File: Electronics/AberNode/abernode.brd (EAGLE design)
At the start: 100 x 80 mm, 12 parts, among them IC1 MCP1703CB, Y1 16MHZ, Y2 16MHZ

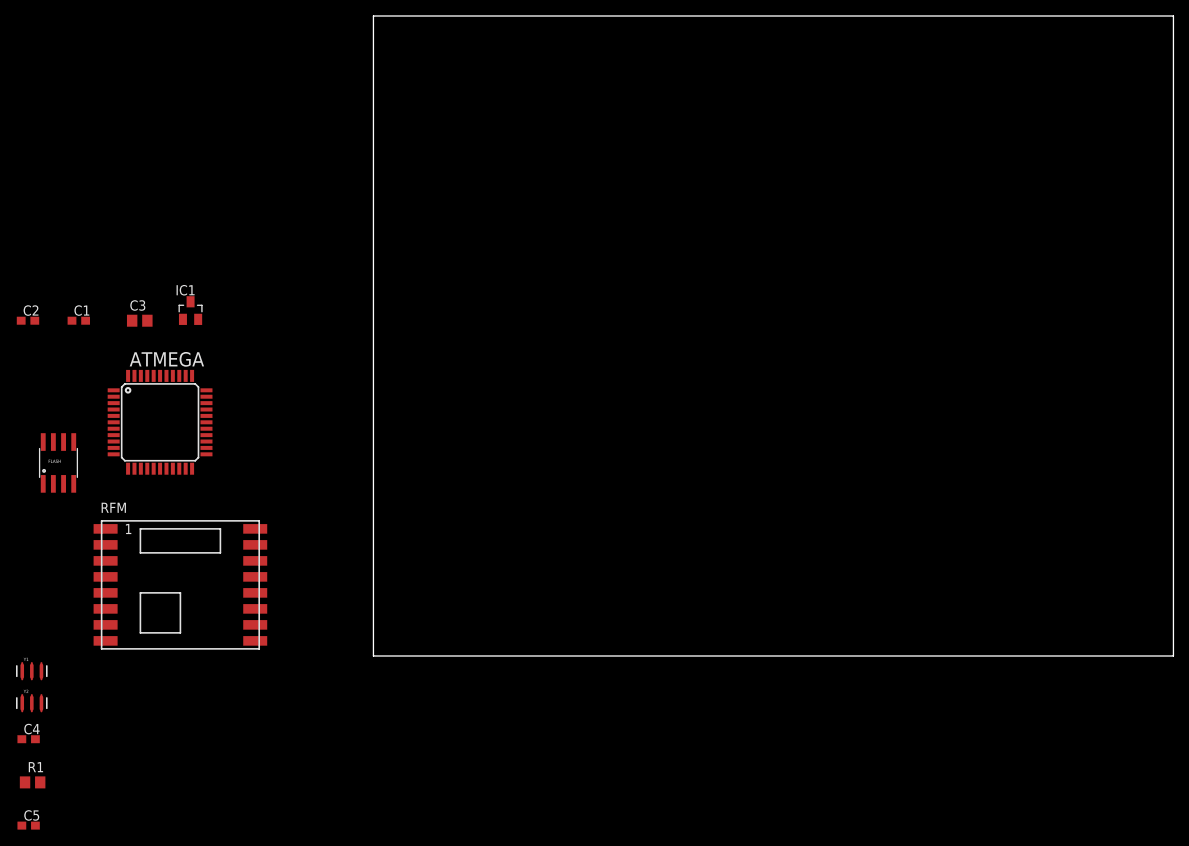
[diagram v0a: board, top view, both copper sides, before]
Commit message: Schematic Mostly Done
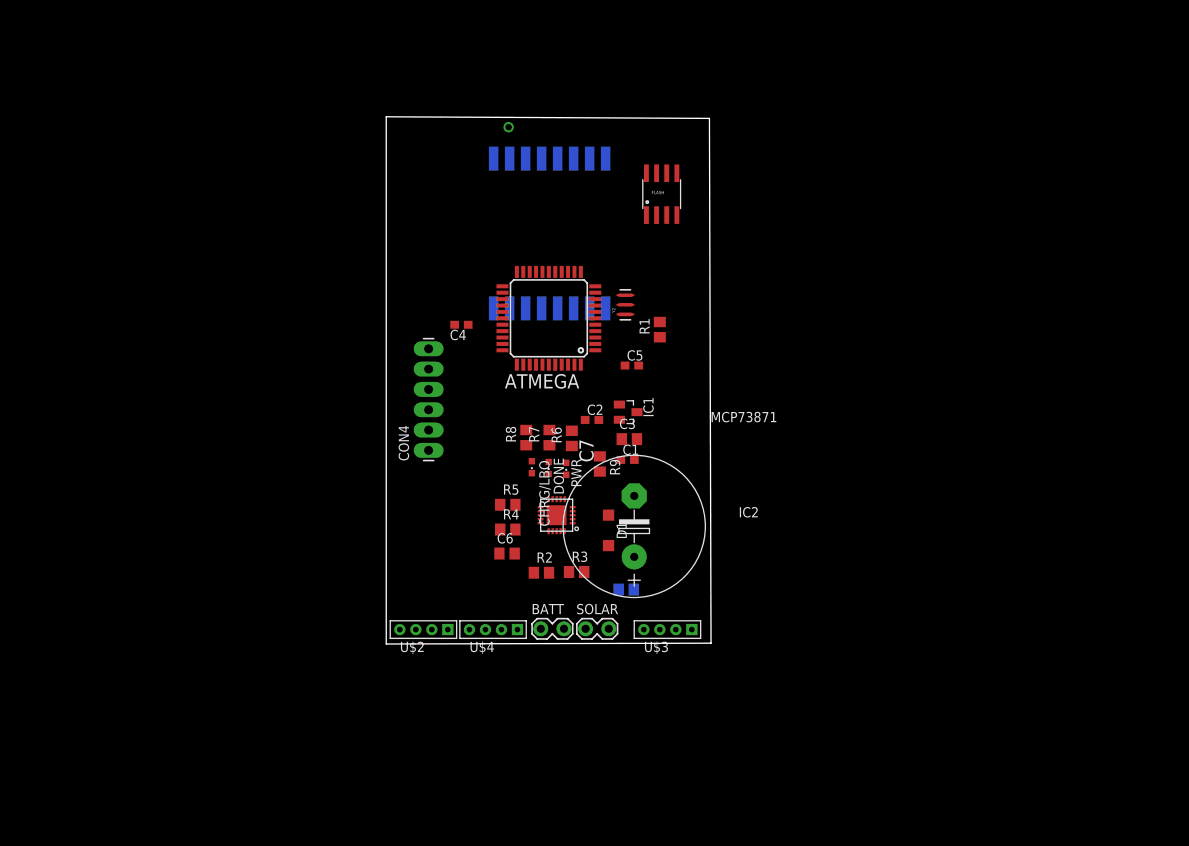
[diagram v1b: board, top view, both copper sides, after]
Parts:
- removed Y1: 16MHZ, SparkFun-FreqCtrl:RESONATOR-SMD
- added BATT, SOLAR: M02LOCK, SparkFun-Connectors:1X02_LOCK
- added C6, C9: 10uF, resistor:C0805
- added C7: (no value), resistor:E7,5-18
- added CHRG/LBO: ORANGE, led:CHIPLED_0603
- added CON4: (no value), SparkFun-Connectors:1X06_LONGPADS
- added D1: MBR0520LT, diode:SOD123
- added DONE: GREEN, led:CHIPLED_0603
- added IC2: MCP73871, adafruit:QFN20
- added PWR: RED, led:CHIPLED_0603
- added R2, R3, R9: 10k, resistor:R0805
- added R4: 2K, resistor:R0805
- added R5: 100K, resistor:R0805
- added R6, R7, R8: 1K, resistor:R0805
- added U$1: (no value), tom:ANT
- added U$2, U$3, U$4: HEADER_4, tom:HEADER_4
- moved R1 96.7 mm to (35.8, 40.8), turned to 90 degrees
- moved C5 94.8 mm to (32.3, 36.3)
- moved Y2 89.4 mm to (31.5, 43.9), turned to 90 degrees
- moved FLASH 82.5 mm to (36.0, 57.7)
- moved C4 74.9 mm to (11.0, 41.4), turned to 180 degrees
- moved C2 71.6 mm to (27.3, 29.5)
- moved C1 70.8 mm to (31.8, 24.5)
- moved RFM 63.7 mm to (22.0, 52.8), flipped to the bottom, turned to 90 degrees
- moved C3 63.0 mm to (32.0, 27.1)
- moved IC1 56.2 mm to (31.8, 30.5), turned to 270 degrees
- moved ATMEGA 50.3 mm to (21.9, 42.2), turned to 180 degrees
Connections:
- removed net PSBATT: C1.2, C3.2, IC1.3
- removed net VCC: C2.2, IC1.2
- new net ANALOG_1: ATMEGA.37, U$2.4
- new net ANALOG_2: ATMEGA.36, U$3.4
- new net ANALOG_3: ATMEGA.35, U$4.4
- new net ANALOG_4: ATMEGA.34, CON4.6
- new net DIGIT_1: ATMEGA.9, U$2.3
- new net DIGIT_2: ATMEGA.10, U$3.3
- new net DIGIT_3: ATMEGA.11, U$4.3
- new net N$10: CHRG/LBO.A, R8.1
- new net N$11: IC2.6, PWR.C
- new net N$12: DONE.C, IC2.7
- new net N$13: CHRG/LBO.C, IC2.8
- new net N$14: D1.A, SOLAR.2
- new net N$17: IC2.5, R9.2
- new net N$5: IC2.12, R5.2
- new net N$6: IC2.2, R2.2, R3.1
- new net N$7: IC2.13, R4.2
- new net N$8: PWR.A, R6.1
- new net N$9: DONE.A, R7.1
- new net SCL: ATMEGA.19, CON4.5
- new net SDA: ATMEGA.20, CON4.4
- new net VBATT: BATT.2, C6.2, IC2.14, IC2.15, IC2.16
- new net VIN: C7.+, C9.2, CON4.2, D1.C, IC2.17, IC2.18, IC2.19, IC2.3, IC2.4, IC2.9, R3.2, R6.2, R7.2, R8.2
- new net VSUPPLY: C1.2, C3.2, IC1.3, IC2.1, IC2.20
- net +3V3: now also C2.2, CON4.1, IC1.2, U$2.2, U$3.2, U$4.2
- net ANT: now also U$1.P$1
- net GND: now also BATT.1, C6.1, C7.-, C9.1, CON4.3, IC2.10, IC2.11, R2.1, R4.1, R5.1, R9.1, SOLAR.1, U$2.1, U$3.1, U$4.1
- net N$3: now also ATMEGA.29
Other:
- board size 100 x 80 mm -> 40.6 x 65.9 mm
